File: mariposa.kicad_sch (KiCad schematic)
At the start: 42 parts, among them J1 Conn_01x28_MountingPin, J3 Conn_ARM_SWD_TagConnect_TC203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, J6 Conn_01x10_MountingPin, J8 Conn_01x04_MountingPin, J9 Conn_02x03_Odd_Even, SW1 SW_Push, SW3 SW_Push

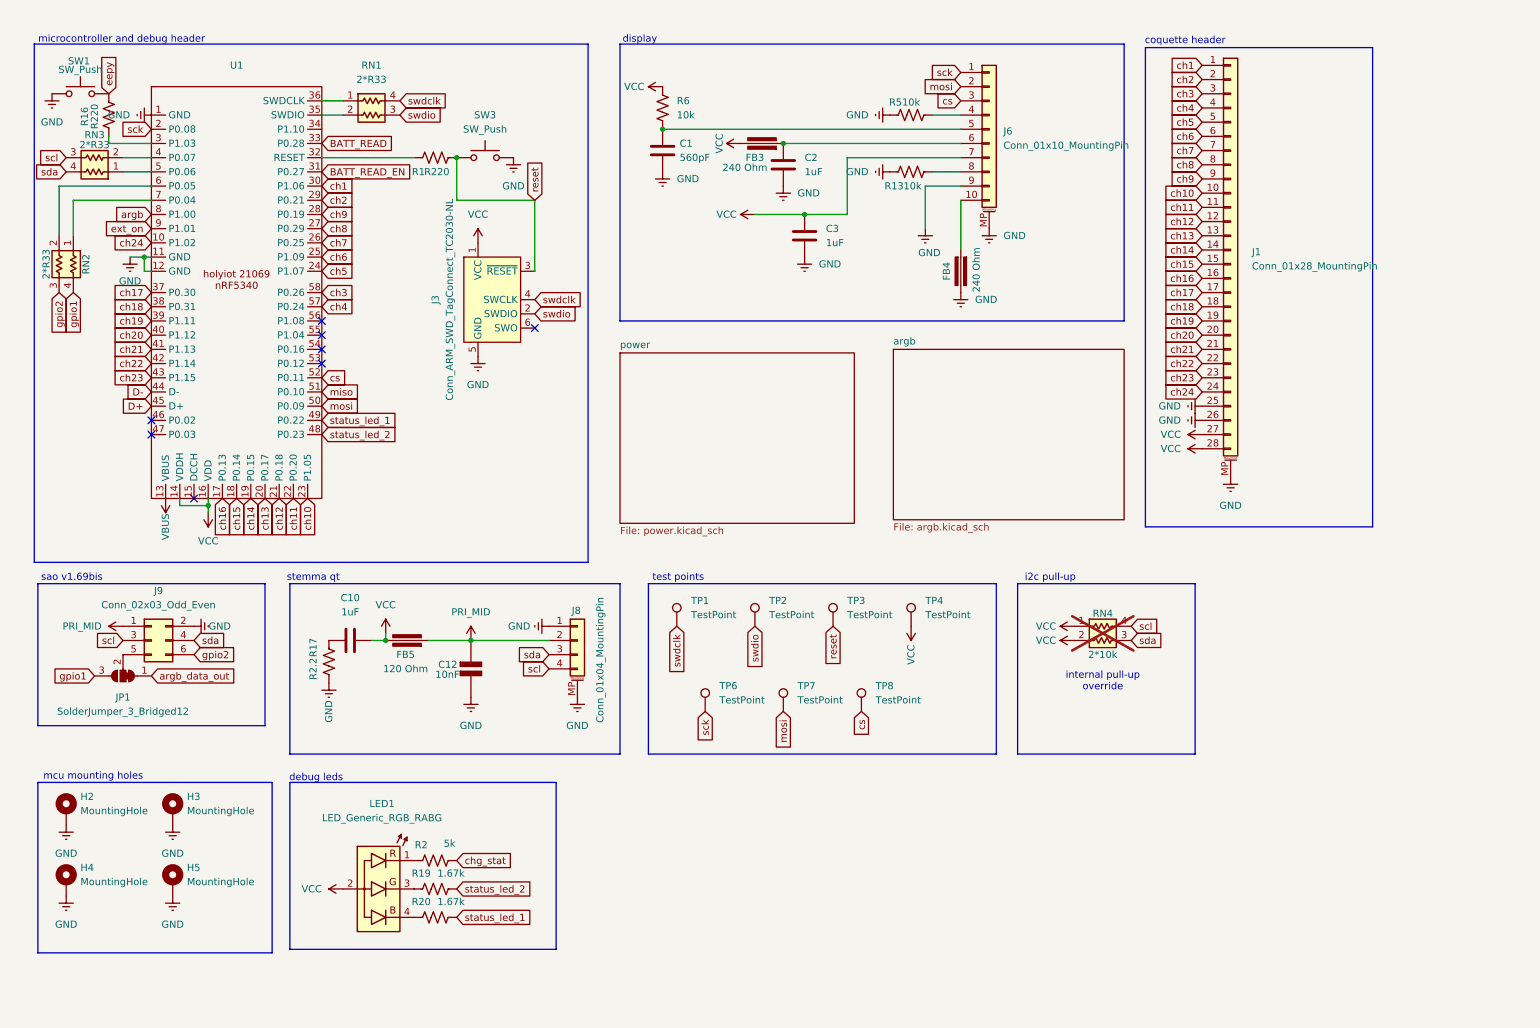
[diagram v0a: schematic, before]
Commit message: v3 efforts
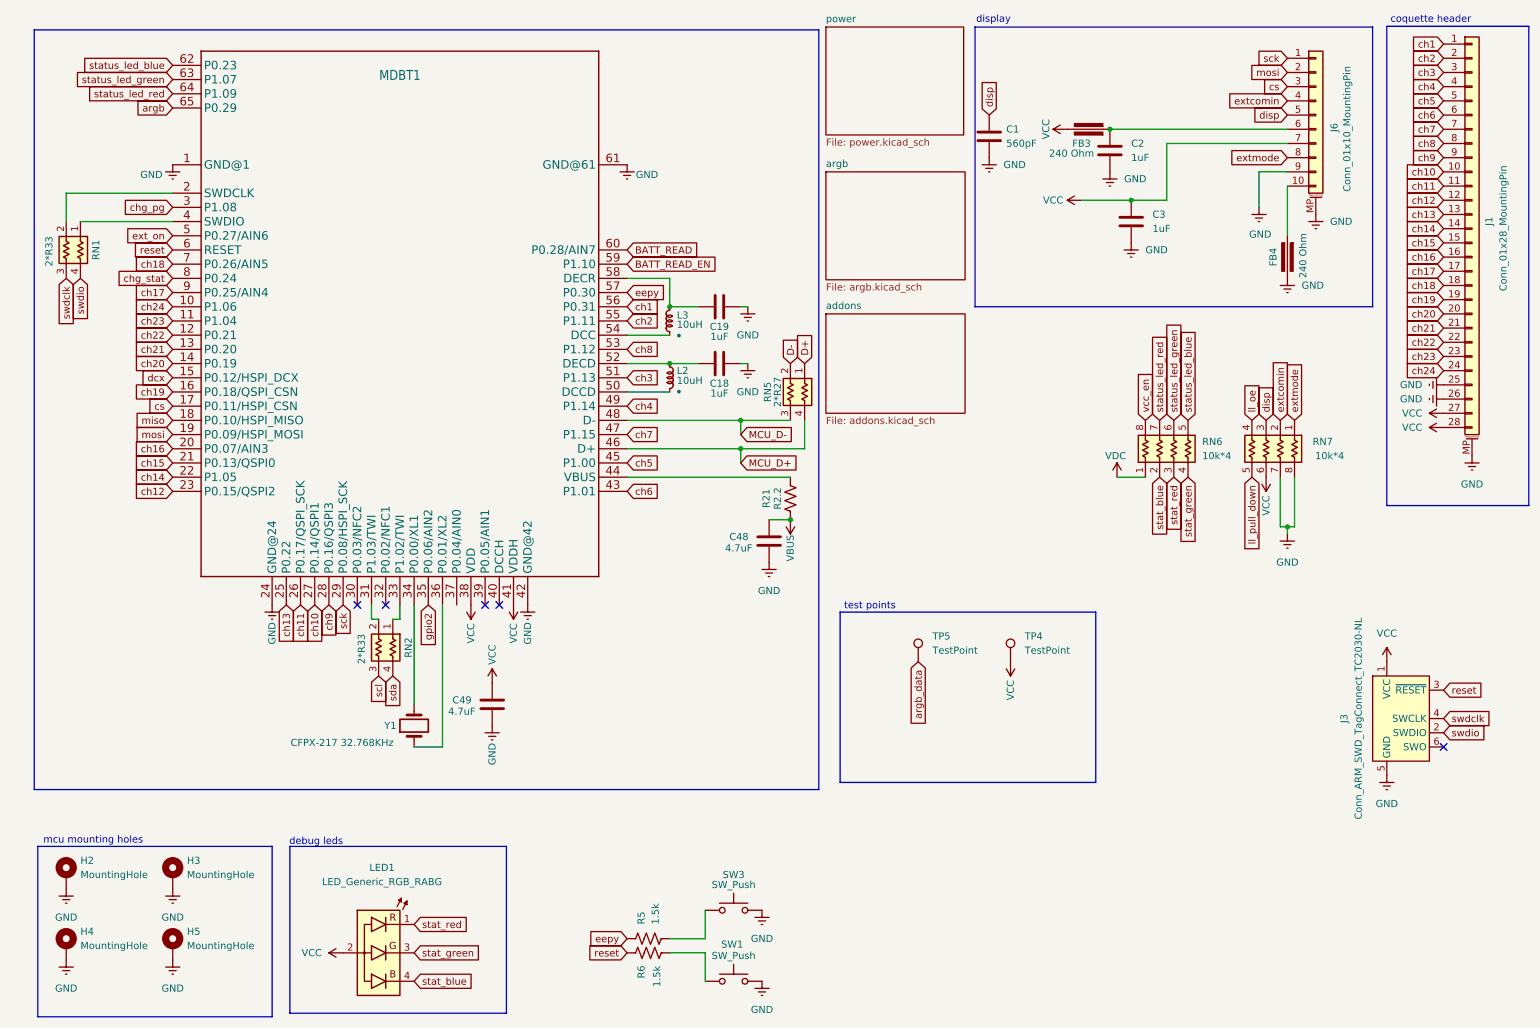
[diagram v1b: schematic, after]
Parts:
- removed C10: 1uF, Capacitor_SMD:C_0603_1608Metric, symbol Device:C
- removed C12: 10nF, Capacitor_SMD:C_0402_1005Metric, symbol PCM_Elektuur:C
- removed FB5: 120 Ohm, PCM_Ferrite_SMD_AKL:Ferrite_0805_2012Metric, symbol PCM_Device_AKL:Ferrite_Bead
- removed J8: Conn_01x04_MountingPin, Connector_JST:JST_SH_SM04B-SRSS-TB_1x04-1MP_P1.00mm_Horizontal, symbol Connector_Generic_MountingPin:Conn_01x04_MountingPin
- removed J9: Conn_02x03_Odd_Even, Connector_PinSocket_2.54mm:PinSocket_2x03_P2.54mm_Vertical_SMD, symbol Connector_Generic:Conn_02x03_Odd_Even
- removed JP1: SolderJumper_3_Bridged12, Jumper:SolderJumper-3_P1.3mm_Bridged12_RoundedPad1.0x1.5mm, symbol Jumper:SolderJumper_3_Bridged12
- removed R1, R16: R220, Resistor_SMD:R_0603_1608Metric, symbol Device:R_US
- removed R13: 10k, Resistor_SMD:R_0603_1608Metric, symbol Device:R_US
- removed R17: R2.2, Resistor_SMD:R_0603_1608Metric, symbol Device:R_US
- removed R19, R20: 1.67k, Resistor_SMD:R_0402_1005Metric, symbol Device:R_US
- removed R2: 5k, Resistor_SMD:R_0402_1005Metric, symbol Device:R_US
- removed RN3: 2*R33, PCM_Resistor_SMD_AKL:R_Array_Convex_2x0402, symbol PCM_Resistor_US_AKL:R_2x0402_Convex
- removed RN4: 2*10k, PCM_Resistor_SMD_AKL:R_Array_Convex_2x0402, symbol PCM_Resistor_US_AKL:R_2x0402_Convex
- removed TP1, TP2, TP3, TP6, TP7, TP8: TestPoint, TestPoint:TestPoint_Pad_D1.0mm, symbol Connector:TestPoint
- removed U1: ~, coquette_footprints:holyiot_21069_nRF5340, symbol coquette_symbols:holyiot_21069_nrf5340
- added C18, C19: 1uF, Capacitor_SMD:C_0603_1608Metric, symbol Device:C
- added C48, C49: 4.7uF, Capacitor_SMD:C_0603_1608Metric, symbol Device:C
- added L2, L3: 10uH, Inductor_SMD:L_0603_1608Metric, symbol PCM_Generic-50:L,IEEE
- added MDBT1: ~, coquette_footprints:MDBT53, symbol coquette_symbols:MDBT53
- added R21: R2.2, Resistor_SMD:R_0603_1608Metric, symbol Device:R_US
- added RN5: 2*R27, Resistor_SMD:R_Array_Convex_2x0603, symbol PCM_Resistor_US_AKL:R_2x0402_Convex
- added RN6, RN7: 10k*4, PCM_Resistor_SMD_AKL:R_Array_Convex_4x0603, symbol PCM_Resistor_US_AKL:R_4x0603_Convex
- added TP5: TestPoint, TestPoint:TestPoint_Pad_D1.0mm, symbol Connector:TestPoint
- added Y1: CFPX-217 32.768KHz, Crystal:Crystal_SMD_3215-2Pin_3.2x1.5mm, symbol Device:Crystal
- J1: footprint coquette_footprints:AMPHENOL_SFV28R-1STE1HLF -> Connector_FFC-FPC:Hirose_FH12-28S-0.5SH_1x28-1MP_P0.50mm_Horizontal
- J6: footprint coquette_footprints:AMPHENOL_SFV10R-1STE1HLF -> Connector_FFC-FPC:Hirose_FH12-10S-0.5SH_1x10-1MP_P0.50mm_Horizontal
- R5, R6: value 10k -> 1.5k
- RN1, RN2: footprint PCM_Resistor_SMD_AKL:R_Array_Convex_2x0402 -> Resistor_SMD:R_Array_Convex_2x0603
- SW1, SW3: footprint Button_Switch_SMD:SW_SPST_PTS645 -> coquette_footprints:G-Switch GT-TC041B-H036-L1N
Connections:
- net gpio1 is gone; now on net sda: RN2.4 (R1.2)
- net BATT_READ: now also MDBT1.60 (P0.28/AIN7)
- net BATT_READ_EN: now also MDBT1.59 (P1.10)
- net D+: now also RN5.1 (R1.1)
- net D-: now also RN5.2 (R2.1)
- net GND: now also SW1.2, C18.1, C19.1, C48.1, C49.1, MDBT1.1 (GND@1), MDBT1.24 (GND@24), MDBT1.42 (GND@42), MDBT1.61 (GND@61), RN7.7 (R2.2), RN7.8 (R1.2); no longer R5.1, SW1.1
- net VBUS: now also C48.2, R21.2
- net VCC: now also C49.2, MDBT1.38 (VDD), MDBT1.41 (VDDH), RN7.6 (R3.2); no longer R6.2
- net argb: now also MDBT1.65 (P0.29)
- net ch1: now also MDBT1.56 (P0.31)
- net ch10: now also MDBT1.27 (P0.14/QSPI1)
- net ch11: now also MDBT1.26 (P0.17/QSPI_SCK)
- net ch12: now also MDBT1.23 (P0.15/QSPI2)
- net ch13: now also MDBT1.25 (P0.22)
- net ch14: now also MDBT1.22 (P1.05)
- net ch15: now also MDBT1.21 (P0.13/QSPI0)
- net ch16: now also MDBT1.20 (P0.07/AIN3)
- net ch17: now also MDBT1.9 (P0.25/AIN4)
- net ch18: now also MDBT1.7 (P0.26/AIN5)
- net ch19: now also MDBT1.16 (P0.18/QSPI_CSN)
- net ch2: now also MDBT1.55 (P1.11)
- net ch20: now also MDBT1.14 (P0.19)
- net ch21: now also MDBT1.13 (P0.20)
- net ch22: now also MDBT1.12 (P0.21)
- net ch23: now also MDBT1.11 (P1.04)
- net ch24: now also MDBT1.10 (P1.06)
- net ch3: now also MDBT1.51 (P1.13)
- net ch4: now also MDBT1.49 (P1.14)
- net ch5: now also MDBT1.45 (P1.00)
- net ch6: now also MDBT1.43 (P1.01)
- net ch7: now also MDBT1.47 (P1.15)
- net ch8: now also MDBT1.53 (P1.12)
- net ch9: now also MDBT1.28 (P0.16/QSPI3)
- net chg_stat: now also MDBT1.8 (P0.24)
- net cs: now also MDBT1.17 (P0.11/HSPI_CSN)
- net eepy: now also R5.1, MDBT1.57 (P0.30); no longer SW1.2
- net ext_on: now also MDBT1.5 (P0.27/AIN6)
- net gpio2: now also MDBT1.35 (P0.06/AIN2); no longer RN2.3 (R2.2)
- net miso: now also MDBT1.18 (P0.10/HSPI_MISO)
- net mosi: now also MDBT1.19 (P0.09/HSPI_MOSI)
- net reset: now also R6.1, MDBT1.6 (RESET); no longer SW3.1
- net sck: now also MDBT1.29 (P0.08/HSPI_SCK)
- net scl: now also RN2.3 (R2.2)
- net swdclk: now also RN1.3 (R2.2); no longer RN1.4 (R1.2)
- net swdio: now also RN1.4 (R1.2); no longer RN1.3 (R2.2)
- net stat_red: now reaches LED1.1 (R)
- net stat_red: now also RN6.3 (R3.1)
- net disp: now reaches C1.1, J6.5 (Pin_5)
- net disp: now also RN7.3 (R3.1); no longer R6.1
- net at R5.2: now also SW3.1; no longer J6.4 (Pin_4)
- net at RN2.1 (R1.1): now also MDBT1.33 (P1.02/TWI)
- net at RN2.2 (R2.1): now also MDBT1.31 (P1.03/TWI)
- net at RN1.1 (R1.1): now also MDBT1.4 (SWDIO)
- net at RN1.2 (R2.1): now also MDBT1.2 (SWDCLK)
- net stat_green: now reaches LED1.3 (G)
- net stat_green: now also RN6.4 (R4.1)
- net stat_blue: now reaches LED1.4 (B)
- net stat_blue: now also RN6.2 (R2.1)
- net extmode: now reaches J6.8 (Pin_8)
- net extmode: now also RN7.1 (R1.1)
- new net: C18.2, L2.1 (+), MDBT1.52 (DECD)
- new net: L2.2 (-), MDBT1.50 (DCCD)
- new net: R6.2, SW1.1
- new net: MDBT1.36 (P0.01/XL2), Y1.1
- new net: MDBT1.34 (P0.00/XL1), Y1.2
- new net: L3.1 (+), MDBT1.54 (DCC)
- new net: C19.2, L3.2 (-), MDBT1.58 (DECR)
- new net: MDBT1.44 (VBUS), R21.1
- new net MCU_D+: MDBT1.46 (D+), RN5.4 (R1.2)
- new net MCU_D-: MDBT1.48 (D-), RN5.3 (R2.2)
- new net VDC: RN6.1 (R1.1)
- new net argb_data: TP5.1
- new net chg_pg: MDBT1.3 (P1.08)
- new net dcx: MDBT1.15 (P0.12/HSPI_DCX)
- new net extcomin: J6.4 (Pin_4), RN7.2 (R2.1)
- new net ll_oe: RN7.4 (R4.1)
- new net ll_pull_down: RN7.5 (R4.2)
- new net status_led_blue: MDBT1.62 (P0.23), RN6.5 (R4.2)
- new net status_led_green: MDBT1.63 (P1.07), RN6.6 (R3.2)
- new net status_led_red: MDBT1.64 (P1.09), RN6.7 (R2.2)
- new net vcc_en: RN6.8 (R1.2)
- no-connect marks 8 -> 5
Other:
- added sheet addons (addons.kicad_sch)
- note removed: "i2c pull-up"
- note removed: "internal pull-up override"
- note removed: "microcontroller and debug header"
- note removed: "sao v1.69bis"
- note removed: "stemma qt"
- moved on the sheet: C1, C2, C3, FB3, FB4, H2, H3, H4, H5, J1, J3, J6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
